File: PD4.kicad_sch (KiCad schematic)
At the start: 16 parts, among them Q33 AO3400A, Q34 AO3400A, Q35 AO3400A, Q36 AO3400A

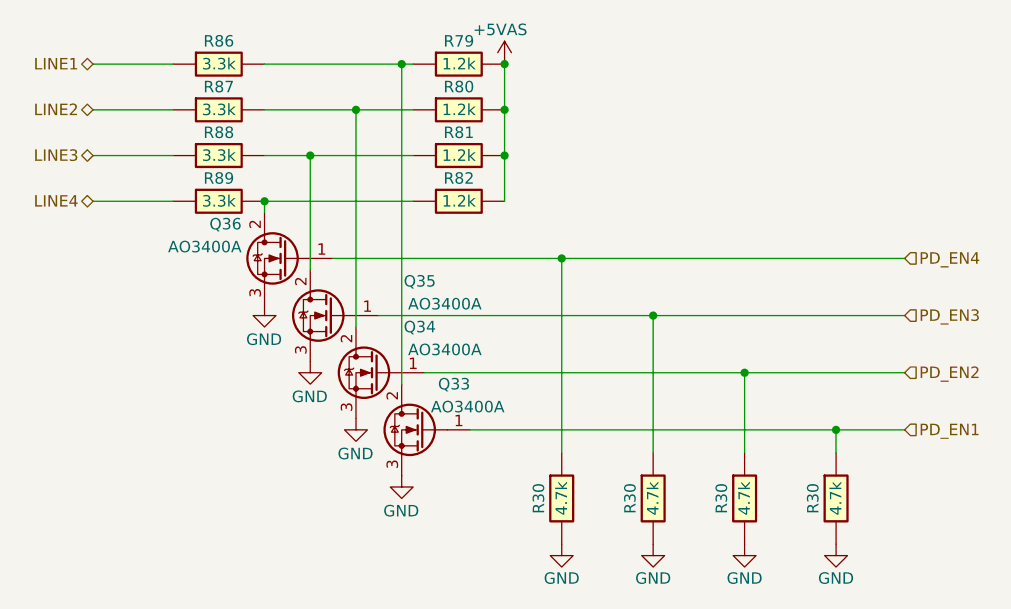
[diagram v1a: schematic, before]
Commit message: Export
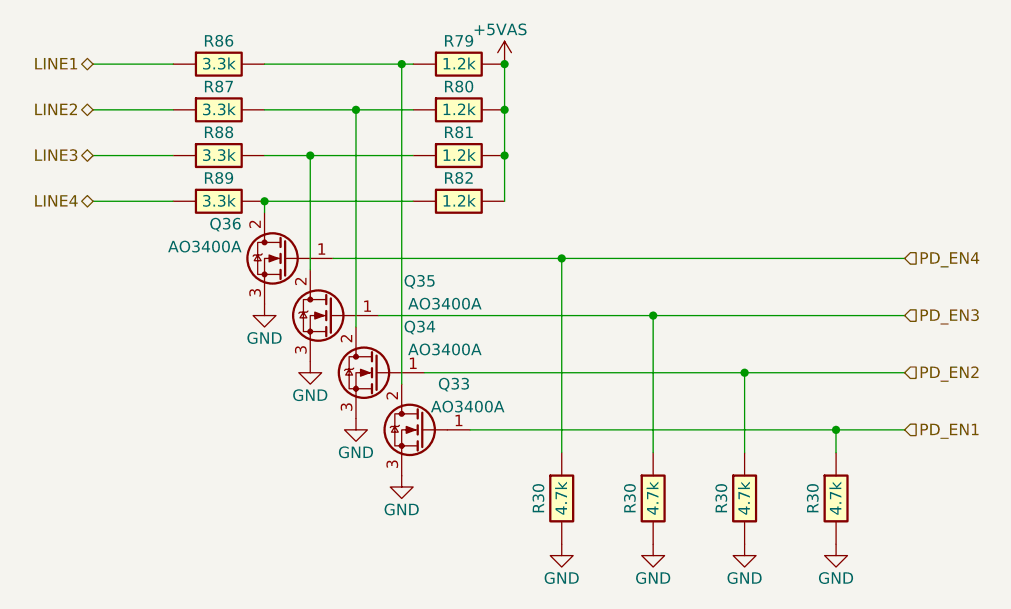
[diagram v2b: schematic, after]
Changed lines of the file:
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@@
       (effects (font (size 1.27 1.27)) hide)
     )
-    (property "Value" "GND" (at 143.4592 130.9434 0)
+    (property "Value" "GND" (at 143.51 130.81 0)
       (effects (font (size 1.27 1.27)))
     )
@@
         )
         (path "/63d2dd9f-d5ff-4811-a88d-0ba932475460/412bf297-30e6-460d-bde0-a70018b48e80"
-          (reference "#PWR0153") (unit 1)
+          (reference "#PWR0209") (unit 1)
         )
       )
@@
       (effects (font (size 1.27 1.27)) hide)
     )
-    (property "Value" "GND" (at 138.3792 124.5934 0)
+    (property "Value" "GND" (at 138.43 124.46 0)
       (effects (font (size 1.27 1.27)))
     )
@@
         )
         (path "/63d2dd9f-d5ff-4811-a88d-0ba932475460/412bf297-30e6-460d-bde0-a70018b48e80"
-          (reference "#PWR0152") (unit 1)
+          (reference "#PWR0210") (unit 1)
         )
       )
@@
       (effects (font (size 1.27 1.27)) hide)
     )
-    (property "Value" "GND" (at 148.5392 137.2934 0)
+    (property "Value" "GND" (at 148.59 137.16 0)
       (effects (font (size 1.27 1.27)))
     )
@@
         )
         (path "/63d2dd9f-d5ff-4811-a88d-0ba932475460/412bf297-30e6-460d-bde0-a70018b48e80"
-          (reference "#PWR0154") (unit 1)
+          (reference "#PWR0207") (unit 1)
         )
       )
@@
       (effects (font (size 1.27 1.27)) hide)
     )
-    (property "Value" "GND" (at 153.6192 143.6434 0)
+    (property "Value" "GND" (at 153.67 143.51 0)
       (effects (font (size 1.27 1.27)))
     )
@@
         )
         (path "/63d2dd9f-d5ff-4811-a88d-0ba932475460/412bf297-30e6-460d-bde0-a70018b48e80"
-          (reference "#PWR0155") (unit 1)
+          (reference "#PWR0208") (unit 1)
         )
       )
@@
         )
         (path "/63d2dd9f-d5ff-4811-a88d-0ba932475460/412bf297-30e6-460d-bde0-a70018b48e80"
-          (reference "#PWR0159") (unit 1)
+          (reference "#PWR0205") (unit 1)
         )
       )
@@
         )
         (path "/63d2dd9f-d5ff-4811-a88d-0ba932475460/412bf297-30e6-460d-bde0-a70018b48e80"
-          (reference "#PWR0158") (unit 1)
+          (reference "#PWR0206") (unit 1)
         )
       )
@@
         )
         (path "/63d2dd9f-d5ff-4811-a88d-0ba932475460/412bf297-30e6-460d-bde0-a70018b48e80"
-          (reference "#PWR0156") (unit 1)
+          (reference "#PWR0203") (unit 1)
         )
       )
@@
         )
         (path "/63d2dd9f-d5ff-4811-a88d-0ba932475460/412bf297-30e6-460d-bde0-a70018b48e80"
-          (reference "#PWR0157") (unit 1)
-        )
-      )
+          (reference "#PWR0204") (unit 1)
+        )
+      )
